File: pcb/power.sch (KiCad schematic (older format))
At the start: 7 parts, among them U6 ADP2108AUJ-3.3

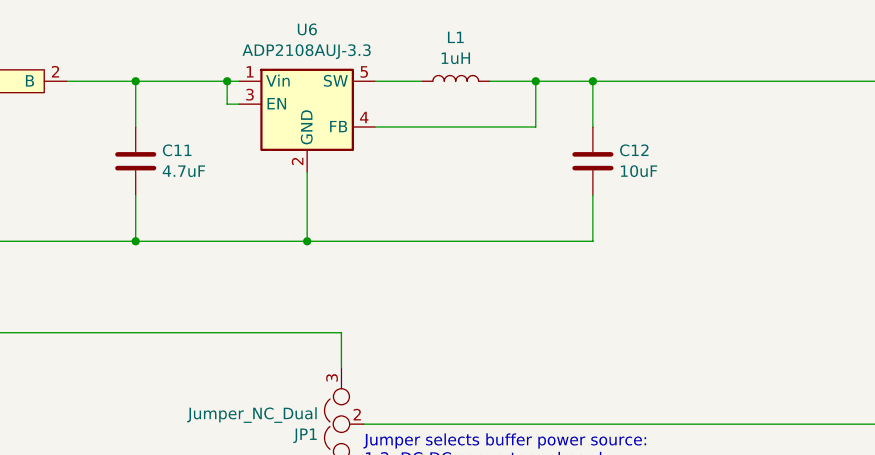
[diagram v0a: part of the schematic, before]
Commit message: more footprints assigned, caps added into open collector base circuit
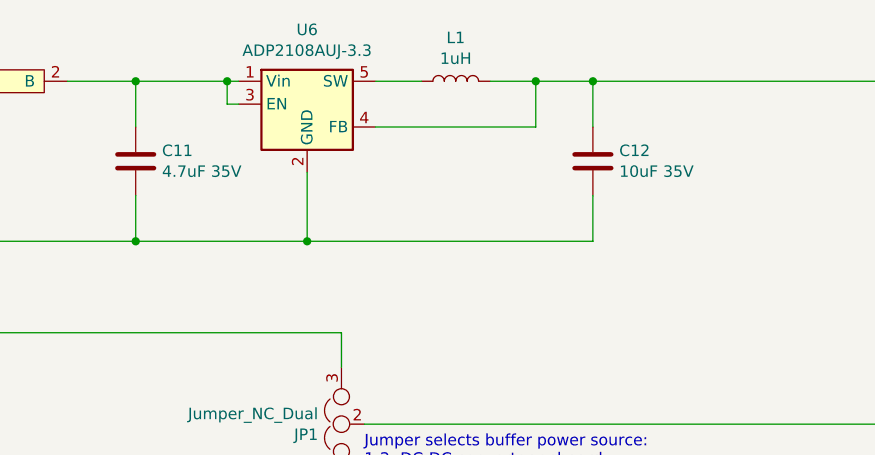
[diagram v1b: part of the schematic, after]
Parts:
- C11: value 4.7uF -> 4.7uF 35V; footprint (none) -> Capacitor_SMD:C_1210_3225Metric_Pad1.42x2.65mm_HandSolder
- C12: value 10uF -> 10uF 35V; footprint (none) -> Capacitor_SMD:C_1210_3225Metric_Pad1.42x2.65mm_HandSolder
- L1: footprint (none) -> Inductor_SMD:L_0603_1608Metric_Pad1.05x0.95mm_HandSolder
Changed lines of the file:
@@
 P 3000 2350
 F 0 "C11" H 3115 2396 50  0000 L CNN
-F 1 "4.7uF" H 3115 2305 50  0000 L CNN
-F 2 "" H 3038 2200 50  0001 C CNN
+F 1 "4.7uF 35V" H 3115 2305 50  0000 L CNN
+F 2 "Capacitor_SMD:C_1210_3225Metric_Pad1.42x2.65mm_HandSolder" H 3038 2200 50  0001 C CNN
 F 3 "~" H 3000 2350 50  0001 C CNN
 	1    3000 2350
@@
 P 5000 2350
 F 0 "C12" H 5115 2396 50  0000 L CNN
-F 1 "10uF" H 5115 2305 50  0000 L CNN
-F 2 "" H 5038 2200 50  0001 C CNN
+F 1 "10uF 35V" H 5115 2305 50  0000 L CNN
+F 2 "Capacitor_SMD:C_1210_3225Metric_Pad1.42x2.65mm_HandSolder" H 5038 2200 50  0001 C CNN
 F 3 "~" H 5000 2350 50  0001 C CNN
 	1    5000 2350
@@
 F 0 "L1" V 4590 2000 50  0000 C CNN
 F 1 "1uH" V 4499 2000 50  0000 C CNN
-F 2 "" H 4400 2000 50  0001 C CNN
+F 2 "Inductor_SMD:L_0603_1608Metric_Pad1.05x0.95mm_HandSolder" H 4400 2000 50  0001 C CNN
 F 3 "~" H 4400 2000 50  0001 C CNN
 	1    4400 2000

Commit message: working on pcb
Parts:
- JP1: footprint Connector_PinSocket_2.54mm:PinSocket_1x03_P2.54mm_Vertical -> Connector_PinHeader_2.54mm:PinHeader_1x03_P2.54mm_Vertical
- JP2: footprint Connector_PinSocket_2.54mm:PinSocket_1x02_P2.54mm_Vertical -> Connector_PinHeader_2.54mm:PinHeader_1x02_P2.54mm_Vertical
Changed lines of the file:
@@
 F 0 "JP1" V 3854 3602 50  0000 L CNN
 F 1 "Jumper_NC_Dual" V 3945 3602 50  0000 L CNN
-F 2 "Connector_PinSocket_2.54mm:PinSocket_1x03_P2.54mm_Vertical" H 3900 3500 50  0001 C CNN
+F 2 "Connector_PinHeader_2.54mm:PinHeader_1x03_P2.54mm_Vertical" H 3900 3500 50  0001 C CNN
 F 3 "~" H 3900 3500 50  0001 C CNN
 	1    3900 3500
@@
 F 0 "JP2" H 3900 4764 50  0000 C CNN
 F 1 "Jumper" H 3900 4673 50  0000 C CNN
-F 2 "Connector_PinSocket_2.54mm:PinSocket_1x02_P2.54mm_Vertical" H 3900 4500 50  0001 C CNN
+F 2 "Connector_PinHeader_2.54mm:PinHeader_1x02_P2.54mm_Vertical" H 3900 4500 50  0001 C CNN
 F 3 "~" H 3900 4500 50  0001 C CNN
 	1    3900 4500
